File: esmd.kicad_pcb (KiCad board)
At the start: 2 copper layers, 30 x 25 mm, 8 parts, among them J1 Conn_01x04, J2 Conn_01x08, J3 Conn_01x02, J4 Conn_01x02, U2 LM78M05_TO252, U3 74HC245

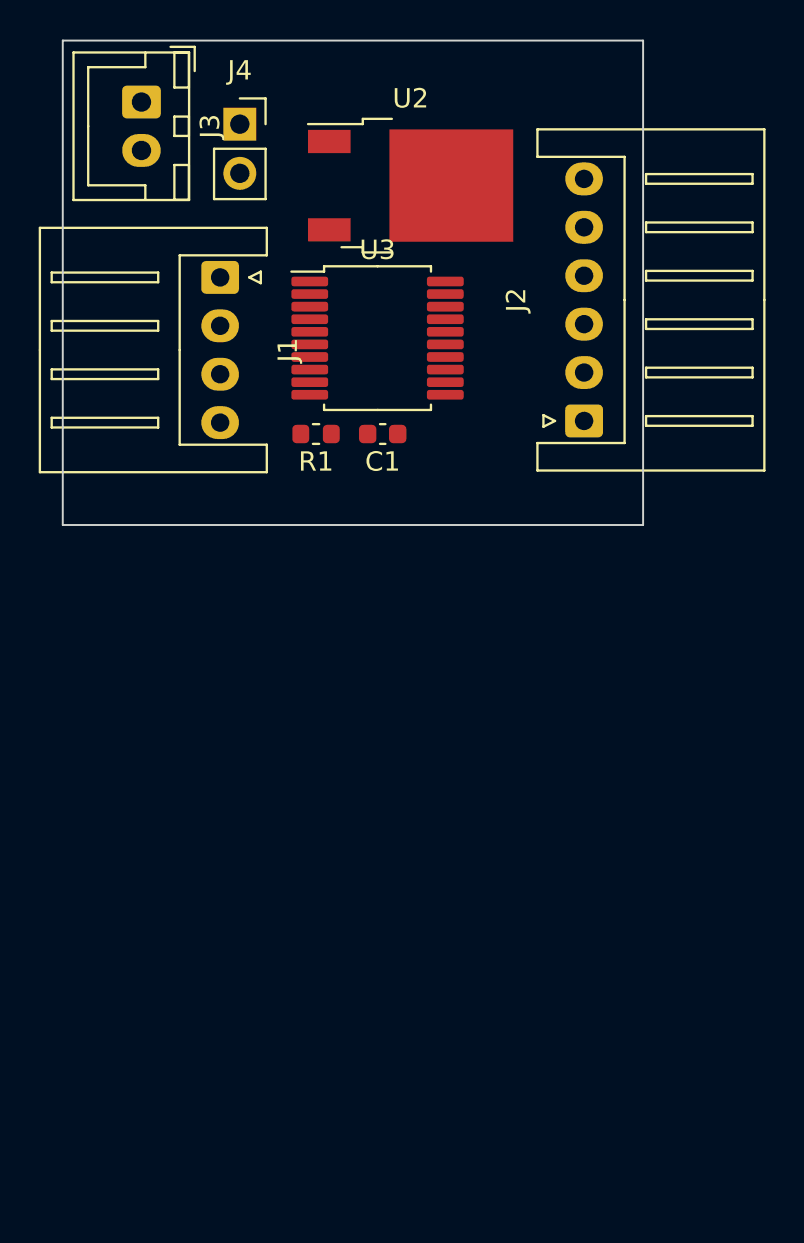
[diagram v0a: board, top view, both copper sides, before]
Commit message: Make it triple.
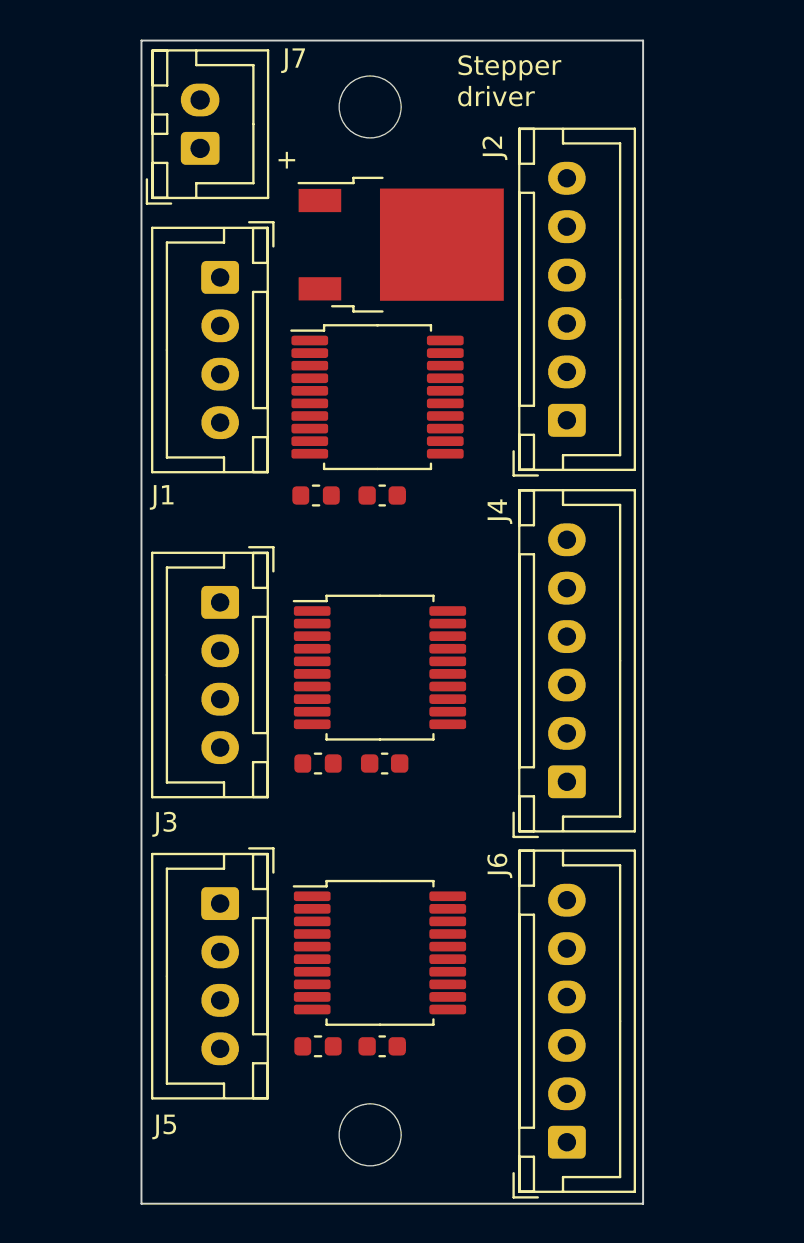
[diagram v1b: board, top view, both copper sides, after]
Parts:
- added C2: 100n, Capacitor_SMD:C_0603_1608Metric, F.Cu at (168.0, 120.0)
- added C3: 100n, Capacitor_SMD:C_0603_1608Metric, F.Cu at (167.9, 134.6)
- added H1: MountingHole, MountingHole:MountingHole_3.2mm_M3, F.Cu at (167.3, 86.1)
- added H2: MountingHole, MountingHole:MountingHole_3.2mm_M3, F.Cu at (167.3, 139.2)
- added J5: Conn_01x04, Connector_JST:JST_XH_B4B-XH-A_1x04_P2.50mm_Vertical, F.Cu at (159.5, 127.2)
- added J6: Conn_01x08, Connector_JST:JST_XH_B6B-XH-A_1x06_P2.50mm_Vertical, F.Cu at (177.4, 139.6)
- added J7: Conn_01x02, Connector_JST:JST_XH_B2B-XH-A_1x02_P2.50mm_Vertical, F.Cu at (158.5, 88.2)
- added R2: 1k, Resistor_SMD:R_0603_1608Metric, F.Cu at (164.6, 120.0)
- added R3: 1k, Resistor_SMD:R_0603_1608Metric, F.Cu at (164.6, 134.6)
- added U1: 74HC245, Package_SO:SSOP-20_5.3x7.2mm_P0.65mm, F.Cu at (167.8, 115.1)
- added U4: 74HC245, Package_SO:SSOP-20_5.3x7.2mm_P0.65mm, F.Cu at (167.8, 129.8)
- J1: footprint Connector_JST:JST_XH_S4B-XH-A_1x04_P2.50mm_Horizontal -> Connector_JST:JST_XH_B4B-XH-A_1x04_P2.50mm_Vertical
- J2: footprint Connector_JST:JST_XH_S6B-XH-A_1x06_P2.50mm_Horizontal -> Connector_JST:JST_XH_B6B-XH-A_1x06_P2.50mm_Vertical
- J3: value Conn_01x02 -> Conn_01x04; footprint Connector_JST:JST_XH_B2B-XH-A_1x02_P2.50mm_Vertical -> Connector_JST:JST_XH_B4B-XH-A_1x04_P2.50mm_Vertical
- J4: value Conn_01x02 -> Conn_01x08; footprint Connector_PinSocket_2.54mm:PinSocket_1x02_P2.54mm_Vertical -> Connector_JST:JST_XH_B6B-XH-A_1x06_P2.50mm_Vertical
- moved J4 37.9 mm to (177.4, 121.0), turned to 90 degrees
- moved J3 26.2 mm to (159.5, 111.7)
- moved C1 3.18 mm to (167.9, 106.2)
- moved R1 3.17 mm to (164.5, 106.2)
- moved U2 3.09 mm to (168.9, 93.2)
- moved U3 3.05 mm to (167.6, 101.1)
- moved J2 0.89 mm to (177.4, 102.3)
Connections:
- net Dir renamed Dir1
- net Dir_out renamed Dir_out1
- net Enable renamed Enable1
- net Enable_out renamed Enable_out1
- net Step renamed Step1
- net Step_out renamed Step_out1
- J3 pad 1: Net-(J3-Pin_1) -> Enable2
- J3 pad 2: GND -> Step2
- J4 pad 1: Net-(J3-Pin_1) -> Dir_out2
- U2 pad 1: Net-(J3-Pin_1) -> Net-(J7-Pin_1)
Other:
- board size 30 x 25 mm -> 25.9 x 60.1 mm
- board text added: "+"
- board text added: "Stepper driver"
- board text added: "https://github.com/bullestock/externalstepperdriver"
